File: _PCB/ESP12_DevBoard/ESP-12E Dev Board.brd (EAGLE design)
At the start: 70 x 75 mm, 34 parts, among them J1 ZX62-B-5PA(33), Q1 UMH3N, U1 CH340C, U2 5V_REG, U3 3V3_REG

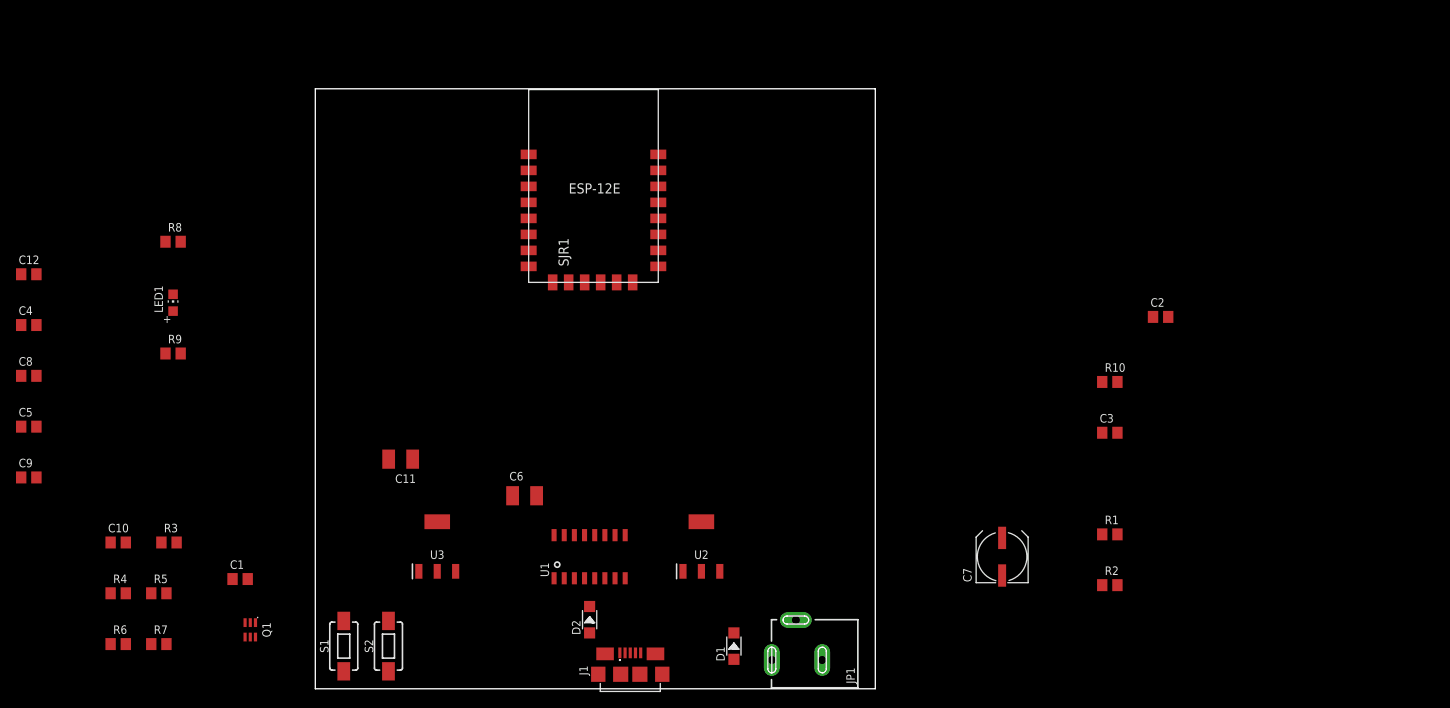
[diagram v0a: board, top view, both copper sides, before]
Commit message: PCB schematic final V1
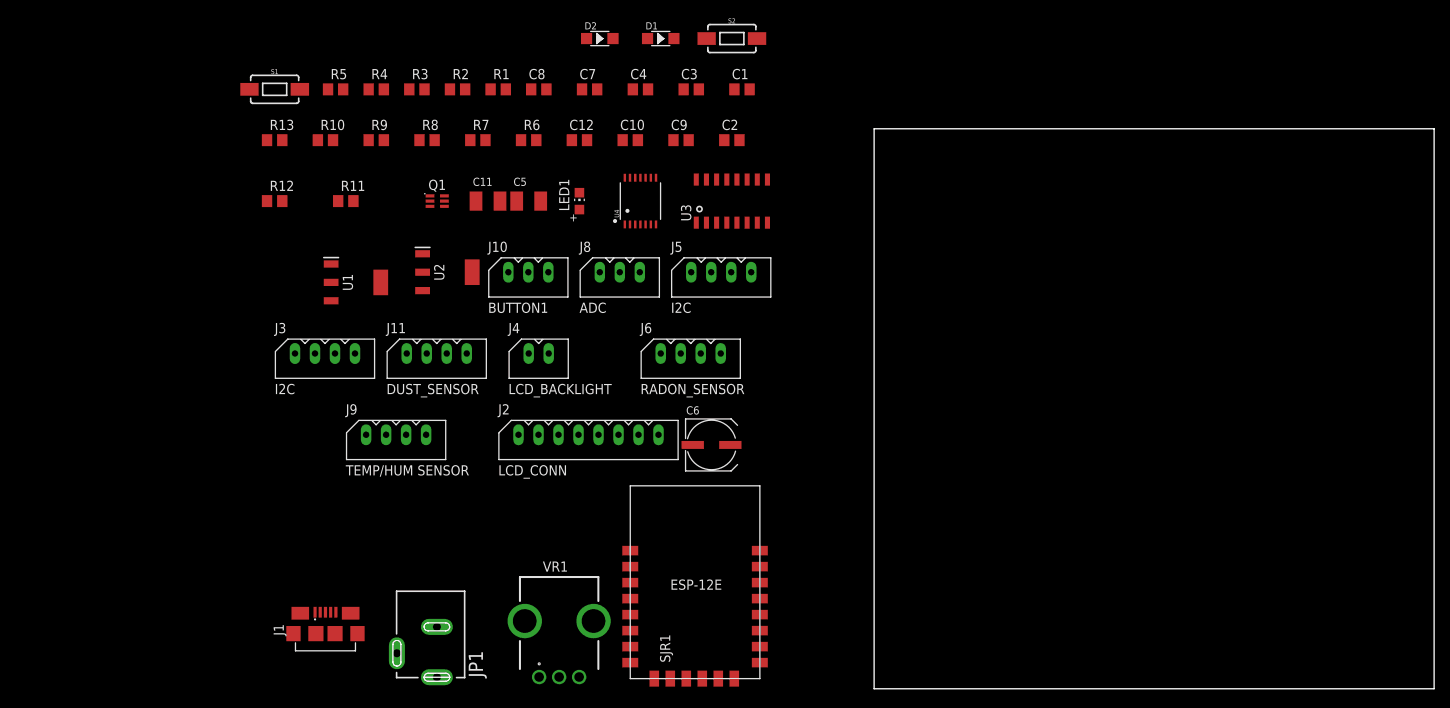
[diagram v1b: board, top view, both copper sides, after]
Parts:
- added J10: BUTTON1, con-molex-spox:5267-3
- added J11: DUST_SENSOR, con-molex-spox:5267-4
- added J2: LCD_CONN, con-molex-spox:5267-8
- added J3, J5: I2C, con-molex-spox:5267-4
- added J4: LCD_BACKLIGHT, con-molex-spox:5267-2
- added J6: RADON_SENSOR, con-molex-spox:5267-4
- added J8: ADC, con-molex-spox:5267-3
- added J9: TEMP/HUM SENSOR, con-molex-spox:5267-4
- added R11: 47k(1%), rcl:R0805
- added R12: 10k(1%), rcl:R0805
- added R13: 470Ω, rcl:R0805
- added U4: TXB0104, SparkFun-IC-Comms:TSSOP14
- added VR1: RK09K1130AAU, SamacSys_Parts:RK09K1130BGM
- C3: value 100nF -> 10uF
- C4, C8: value 10uF -> 22uF
- C5: value 22uF -> 100uF; device rcl:C0805 -> rcl:SMC_B
- C6: value 100uF -> 220uF(optional); device rcl:SMC_B -> rcl:UD-6,3X7,7_NICHICON
- C7: value 220uF -> 10uF; device rcl:UD-6,3X7,7_NICHICON -> rcl:C0805
- C9: value 22uF -> 100nF
- LED1: value blue -> green
- R1, R2: value 470Ω -> 10k
- R6, R7: value 10k -> 470Ω
- U1: value CH340C -> 5V_REG; device ch340g:SOIC16 -> SamacSys_Parts:SOT230P700X170-4N
- U2: value 5V_REG -> 3.3V_REG
- U3: value 3V3_REG -> CH340C; device SamacSys_Parts:SOT230P700X170-4N -> ch340g:SOIC16
- moved R10 102.6 mm to (-68.6, 68.6)
- moved R2 102.4 mm to (-52.1, 74.9)
- moved R1 94.5 mm to (-47.0, 74.9)
- moved C9 91.8 mm to (-24.1, 68.6)
- moved C1 87.7 mm to (-16.5, 74.9)
- moved S2 87.2 mm to (-17.8, 81.3), turned to 0 degrees
- moved C4 81.9 mm to (-29.2, 74.9)
- moved C10 81.4 mm to (-30.5, 68.6)
- moved R6 81.2 mm to (-43.2, 68.6)
- moved C7 77.9 mm to (-35.6, 74.9), turned to 0 degrees
- moved D1 76.5 mm to (-26.7, 81.3), turned to 0 degrees
- moved R7 74.6 mm to (-49.5, 68.6)
- moved C8 73.1 mm to (-41.9, 74.9)
- moved D2 72.7 mm to (-34.3, 81.3), turned to 0 degrees
- moved C12 70.8 mm to (-36.8, 68.6)
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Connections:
- removed net RXD_ESP: SJR1.15
- removed net TXD_ESP: SJR1.16
- new net LED+_5V: J2.P$7, J4.P$2, U4.11
- new net LED-_5V: J2.P$8, U4.10
- new net N$2: J2.P$3, VR1.2
- new net N$6: J6.P$3, R10.2
- new net N$9: J11.P$3, R13.2
- new net SCL_5V: J2.P$4, J3.P$3, J5.P$3, U4.13
- new net SDA_5V: J2.P$5, J3.P$4, J5.P$4, U4.12
- net 12V: now also C3.1, J6.P$2, U1.3; no longer C4.1, U2.3
- net 3.3V: now also C8.2, J10.P$2, J9.P$2, R1.1, R2.1, U2.2, U2.4, U4.1, U4.8; no longer C9.2, R5.1, R8.1, U3.2, U3.4
- net 5V: now also C10.2, C4.1, C5.+, C7.1, J11.P$2, J2.P$2, J3.P$2, J5.P$2, J8.P$2, U1.2, U1.4, U2.3, U3.16, U4.14, VR1.3; no longer C3.2, C5.1, C7.+, C8.1, U1.16, U2.2, U2.4, U3.3
- net ADC: now also R11.1, R12.2
- net D+_USB: now also U3.5; no longer U1.5
- net D-_USB: now also U3.6; no longer U1.6
- net DTR: now also U3.13; no longer U1.13
- net EN: now also R3.2; no longer R5.2
- net GND: now also C3.2, C5.-, C7.2, C8.1, J10.P$1, J11.P$1, J2.P$1, J3.P$1, J4.P$1, J5.P$1, J6.P$1, J8.P$1, J9.P$1, LED1.C, R12.1, R5.1, U4.7, VR1.1; no longer C3.1, C5.2, C7.-, C8.2, R7.1
- net GPIO0: now also R1.2, U4.4; no longer R3.2
- net GPIO12: now also R10.1
- net GPIO13: now also J6.P$4
- net GPIO14: now also R13.1
- net GPIO15: now also J10.P$3, R5.2; no longer R7.2
- net GPIO16: now also J11.P$4, R8.1; no longer LED1.C, R10.1
- net GPIO2: now also R2.2, U4.5; no longer R4.2
- net GPIO4: now also J9.P$4, U4.3
- net GPIO5: now also J9.P$3, U4.2
- net N$1: now also C9.2, U3.4; no longer C2.2, U1.4
- net N$3: now also R9.2, U3.2; no longer R1.2, U1.2
- net N$4: now also R6.2; no longer R8.2
- net N$5: now also J8.P$3, R11.2; no longer R2.2, U1.3
- net POWER: now also R7.2; no longer R9.2
- net POWER1: now also R8.2; no longer R10.2
- net RST: now also C2.2, R4.2, R7.1; no longer C10.2, R6.2, R9.1
- net RTS: now also U3.14; no longer U1.14
- net RXD: now also R9.1, SJR1.15; no longer R1.1
- net TXD: now also SJR1.16, U3.3; no longer R2.1
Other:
- board size 70 x 75 mm -> 70 x 70 mm
